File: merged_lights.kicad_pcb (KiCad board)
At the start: 2 copper layers, 70 x 100 mm, 62 parts, among them J1 Conn_01x08, J2 Conn_01x08, J3 AVR-ISP-6, J4 Conn_01x02, J5 Conn_01x02, J6 Conn_01x02, J7 Conn_01x08, J8 Conn_01x02, J9 Conn_01x08, Q1 AO3400A, Q2 AO3400A, Q3 AO3400A, Q4 AO3400A, Q5 AO3400A, Q6 AO3400A, Q7 AO3400A, Q8 AO3400A, SW1 SW_Push, U1 ATmega328P-A, U2 ADXL345BCCZ

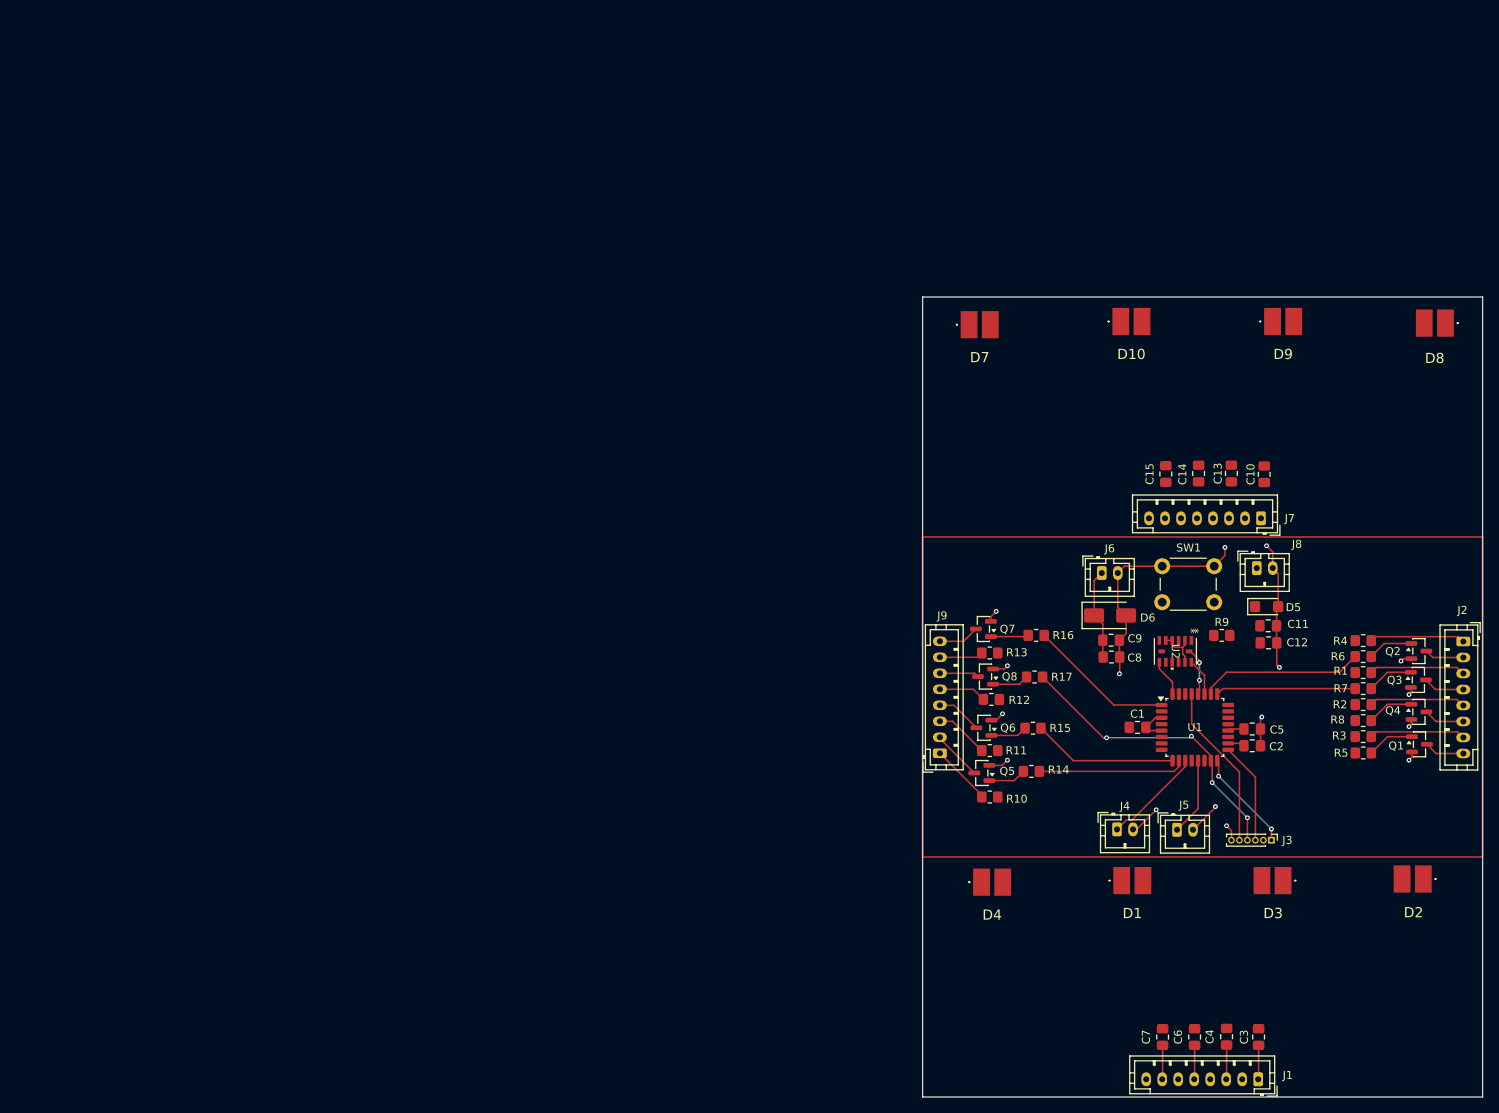
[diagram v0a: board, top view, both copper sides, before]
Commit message: Update merged_lights.kicad_pcb
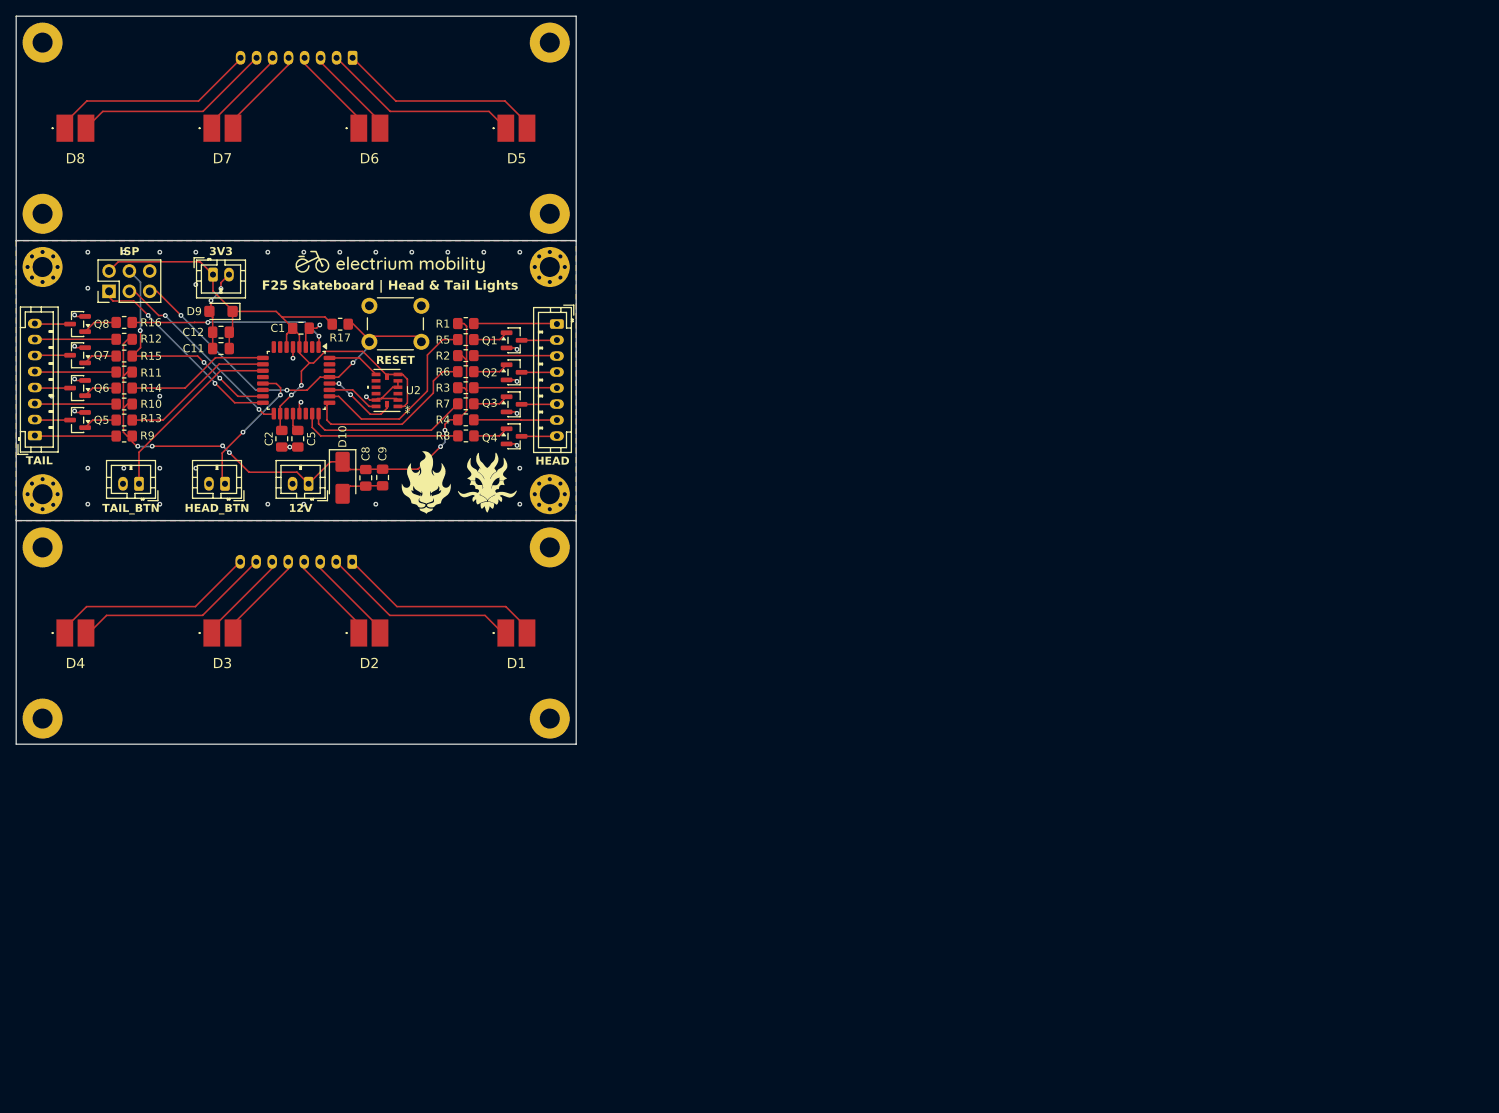
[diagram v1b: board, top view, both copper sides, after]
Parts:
- removed C10, C13, C14, C15, C3, C4, C6, C7: C, Capacitor_SMD:C_0805_2012Metric_Pad1.18x1.45mm_HandSolder
- added G***: LOGO, LOGO, F.Cu at (58.9, 43.0)
- added G***: LOGO, LOGO, F.Cu at (70.9, 70.5)
- added G***: LOGO, LOGO, F.Cu at (63.4, 70.5)
- added G***: LOGO, LOGO, B.Cu at (47.0, 34.0)
- added G***: LOGO, LOGO, B.Cu at (47.0, 88.3)
- added G***: LOGO, LOGO, B.Cu at (47.2, 97.2)
- added G***: LOGO, LOGO, B.Cu at (47.0, 25.2)
- added G***: LOGO, LOGO, B.Cu at (47.0, 56.4)
- added H1: MountingHole_Pad, MountingHole:MountingHole_2.5mm_Pad_Via, F.Cu at (78.8, 43.5)
- added H10: MountingHole_Pad, MountingHole:MountingHole_2.5mm_Pad, F.Cu at (15.4, 36.9)
- added H11: MountingHole_Pad, MountingHole:MountingHole_2.5mm_Pad, F.Cu at (78.8, 100.0)
- added H12: MountingHole_Pad, MountingHole:MountingHole_2.5mm_Pad, F.Cu at (78.8, 36.9)
- added H2: MountingHole_Pad, MountingHole:MountingHole_2.5mm_Pad_Via, F.Cu at (15.4, 43.5)
- added H3: MountingHole_Pad, MountingHole:MountingHole_2.5mm_Pad_Via, F.Cu at (15.4, 72.0)
- added H4: MountingHole_Pad, MountingHole:MountingHole_2.5mm_Pad_Via, F.Cu at (78.8, 72.0)
- added H5: MountingHole_Pad, MountingHole:MountingHole_2.5mm_Pad, F.Cu at (15.4, 78.6)
- added H6: MountingHole_Pad, MountingHole:MountingHole_2.5mm_Pad, F.Cu at (15.4, 100.0)
- added H7: MountingHole_Pad, MountingHole:MountingHole_2.5mm_Pad, F.Cu at (78.8, 78.6)
- added H8: MountingHole_Pad, MountingHole:MountingHole_2.5mm_Pad, F.Cu at (15.4, 15.5)
- added H9: MountingHole_Pad, MountingHole:MountingHole_2.5mm_Pad, F.Cu at (78.8, 15.5)
- J1, J7: moved to B.Cu
- J3: footprint Connector_PinHeader_1.00mm:PinHeader_1x06_P1.00mm_Vertical -> Connector_PinHeader_2.54mm:PinHeader_2x03_P2.54mm_Vertical
- moved J3 160.7 mm to (23.7, 46.6), turned to 90 degrees
- moved C12 136.6 mm to (37.7, 51.7), turned to 180 degrees
- moved D9 135.8 mm to (37.7, 49.1), turned to 180 degrees
- moved J8 135.5 mm to (36.7, 44.5)
- moved C11 135.4 mm to (37.7, 53.7), turned to 180 degrees
- moved J1 130.4 mm to (54.1, 80.4)
- moved J4 129.7 mm to (27.4, 70.7), turned to 180 degrees
- moved J7 127.3 mm to (54.1, 17.4)
- moved C2 127.2 mm to (45.3, 65.0), turned to -90 degrees
- moved J5 126.6 mm to (38.2, 70.7), turned to 180 degrees
- moved C5 124.7 mm to (47.3, 65.0), turned to -90 degrees
- moved R13 121.6 mm to (25.6, 62.7)
- moved Q5 121.3 mm to (19.8, 62.7)
- moved R14 121.3 mm to (25.6, 58.7)
- moved Q6 121.0 mm to (19.8, 58.7)
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- renumbered D2 to D1, D6 to D10, D3 to D2, D1 to D3, D8 to D5, D9 to D6, D10 to D7, D7 to D8, D5 to D9, Q2 to Q1, Q3 to Q2, Q4 to Q3, Q1 to Q4, Q8 to Q7, Q7 to Q8, R4 to R1, R11 to R10, R12 to R11, R13 to R12, R14 to R13, R15 to R14, R17 to R15, R9 to R17, R1 to R2, R2 to R3, R3 to R4, R6 to R5, R7 to R6, R8 to R7, R5 to R8, R10 to R9
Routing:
- net +3.3V: track 2.09 -> 76.3 mm, vias 0 -> 2
- net +12V: track 11.3 -> 81.4 mm, vias 0 -> 6
- net GND: track 81.4 -> 45.1 mm, vias 16 -> 42
- net /TLB4.2: track 0.00 -> 26.5 mm
- net /TLB1.1: track 0.00 -> 26.5 mm
- net /HLB4.2: track 0.00 -> 26.2 mm
- net /TLB4.1: track 0.00 -> 25.0 mm
- net /HLB1.2: track 0.00 -> 24.9 mm
- net /RESET: track 20.7 -> 45.6 mm, vias 0 -> 3
- net /TLB1.2: track 0.00 -> 24.8 mm
- net /HLB1.1: track 4.27 -> 25.9 mm
- net /HLB4.1: track 4.27 -> 25.0 mm
- net /HLED4: track 0.00 -> 20.4 mm
- net /HLED3: track 0.00 -> 20.4 mm
- net Net-(J3-MISO): track 12.7 -> 25.5 mm
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- added copper zone on B.Cu, net GND
- added copper zone on F.Cu, net GND
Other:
- board size 70 x 100 mm -> 70 x 91 mm
- board text added: "12V"
- board text added: "3V3"
- board text added: "F25 Skateboard | Head & Tail Lights"
- board text added: "H1"
- board text added: "H2"
- board text added: "H3"
- board text added: "H4"
- board text added: "HEAD"
- board text added: "HEAD LIGHT"
- board text added: "HEAD_BTN"
- board text added: "Head & Tail Lights Board for F25 Skateboard by Leopoldo Mendoza, Haris Niaz, Catherine Huang"
- board text added: "ISP"
- board text added: "RESET"
- board text added: "T1"
- board text added: "T2"
- board text added: "T3"
- board text added: "T4"
- board text added: "TAIL"
- board text added: "TAIL LIGHT"
- board text added: "TAIL_BTN"
